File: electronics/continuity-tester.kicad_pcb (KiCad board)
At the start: 2 copper layers, 25.4 x 25.4 mm, 14 parts, among them IC1 PIC12LF1571-I/SN, P1 CONN_01X01, P2 CONN_01X01, SW1 SW_PUSH

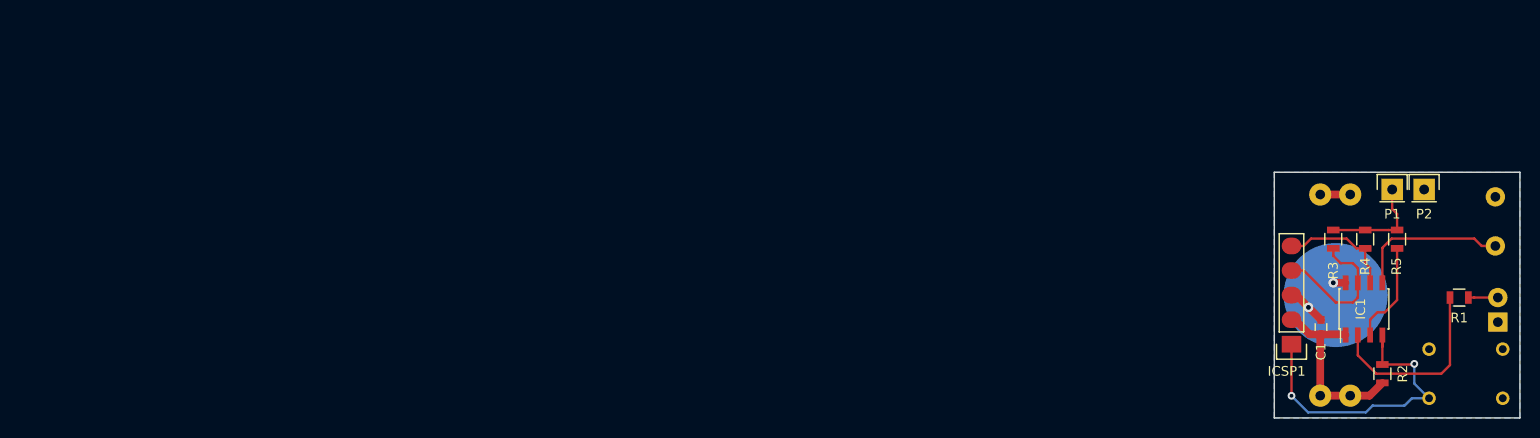
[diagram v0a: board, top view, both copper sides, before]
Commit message: New PCB revision, sent to fab.
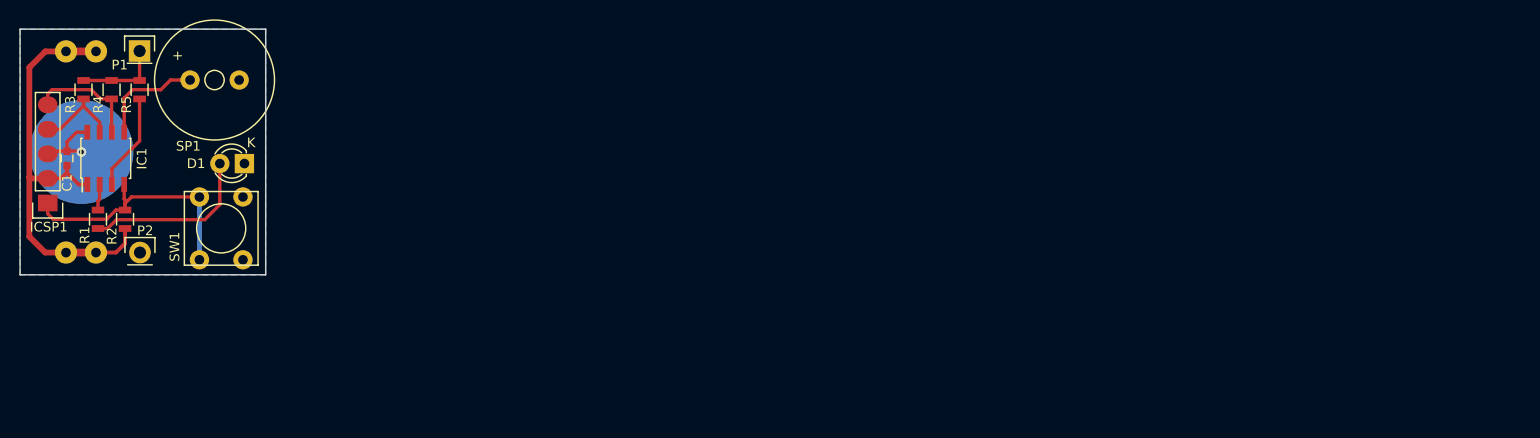
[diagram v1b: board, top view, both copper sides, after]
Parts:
- D1, SP1, SW1: moved to F.Cu
- moved R1 141.0 mm to (71.4, 96.3), turned to 90 degrees
- moved SP1 133.3 mm to (83.4, 81.9), turned to 0 degrees
- moved P2 133.0 mm to (75.7, 99.7)
- moved IC1 131.0 mm to (72.2, 90.0)
- moved R2 131.0 mm to (74.2, 96.3)
- moved R5 131.0 mm to (75.7, 82.9)
- moved C1 130.8 mm to (68.2, 90.0)
- moved D1 130.6 mm to (86.5, 90.5), turned to 180 degrees
- moved R4 130.6 mm to (72.8, 82.9)
- moved BT1 130.5 mm to (69.7, 89.3)
- moved P1 130.3 mm to (75.7, 78.9)
- moved R3 130.2 mm to (69.9, 82.9)
- moved SW1 129.6 mm to (84.1, 97.2), turned to 270 degrees
- moved ICSP1 129.4 mm to (66.2, 94.6)
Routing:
- net Net-(BT1-Pad1): track 22.7 -> 45.8 mm
- net Net-(IC1-Pad2): track 19.8 -> 2.72 mm
- net Net-(D1-Pad2): track 3.05 -> 17.9 mm
- net Net-(IC1-Pad7): track 15.3 -> 9.11 mm
- net Net-(IC1-Pad4): track 32.6 -> 27.6 mm, vias 2 -> 0
- net Net-(IC1-Pad5): track 16.0 -> 11.1 mm
- net Net-(P1-Pad1): track 11.0 -> 8.85 mm
- net Net-(BT1-Pad2): track 5.38 -> 7.11 mm, vias 2 -> 1
- net Net-(IC1-Pad3): track 10.6 -> 10.0 mm
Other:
- net class Default: clearance 0.2 -> 0.25; trace_width 0.25 -> 0.35; via_dia 0.6 -> 0.8
- net class Power: clearance 0.2 -> 0.25; trace_width 0.8 -> 0.4
- rule pad_to_mask_clearance: 0.2 -> 0
- rule trace_clearance: 0.2 -> 0.25
- rule trace_min: 0.2 -> 0.3
- board text added: "LOW POWER CONTINUITY TESTER"
- board text added: "©2015 JIR"
